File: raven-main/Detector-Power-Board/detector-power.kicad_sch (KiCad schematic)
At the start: 34 parts, among them J1 DeployLipo, J2 Conn_01x06, J9 UCLipo, U1 LM51571QRTERQ1, U7 TPS7A4701xRGW, U8 TPS7A4701xRGW

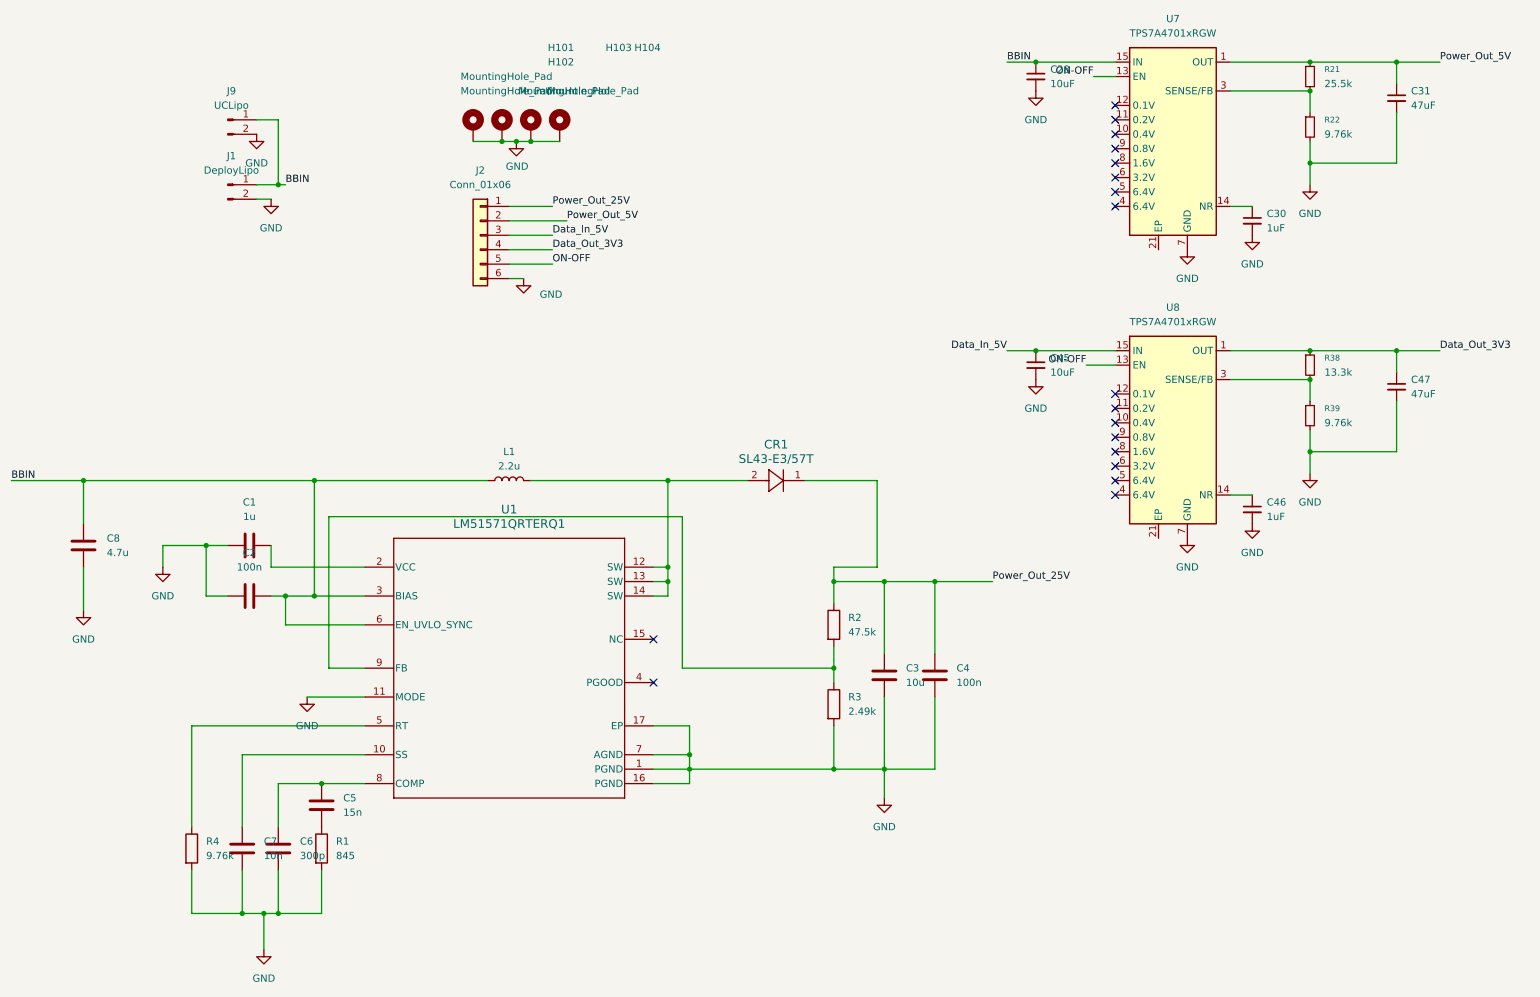
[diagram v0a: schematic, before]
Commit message: Updated power circuit
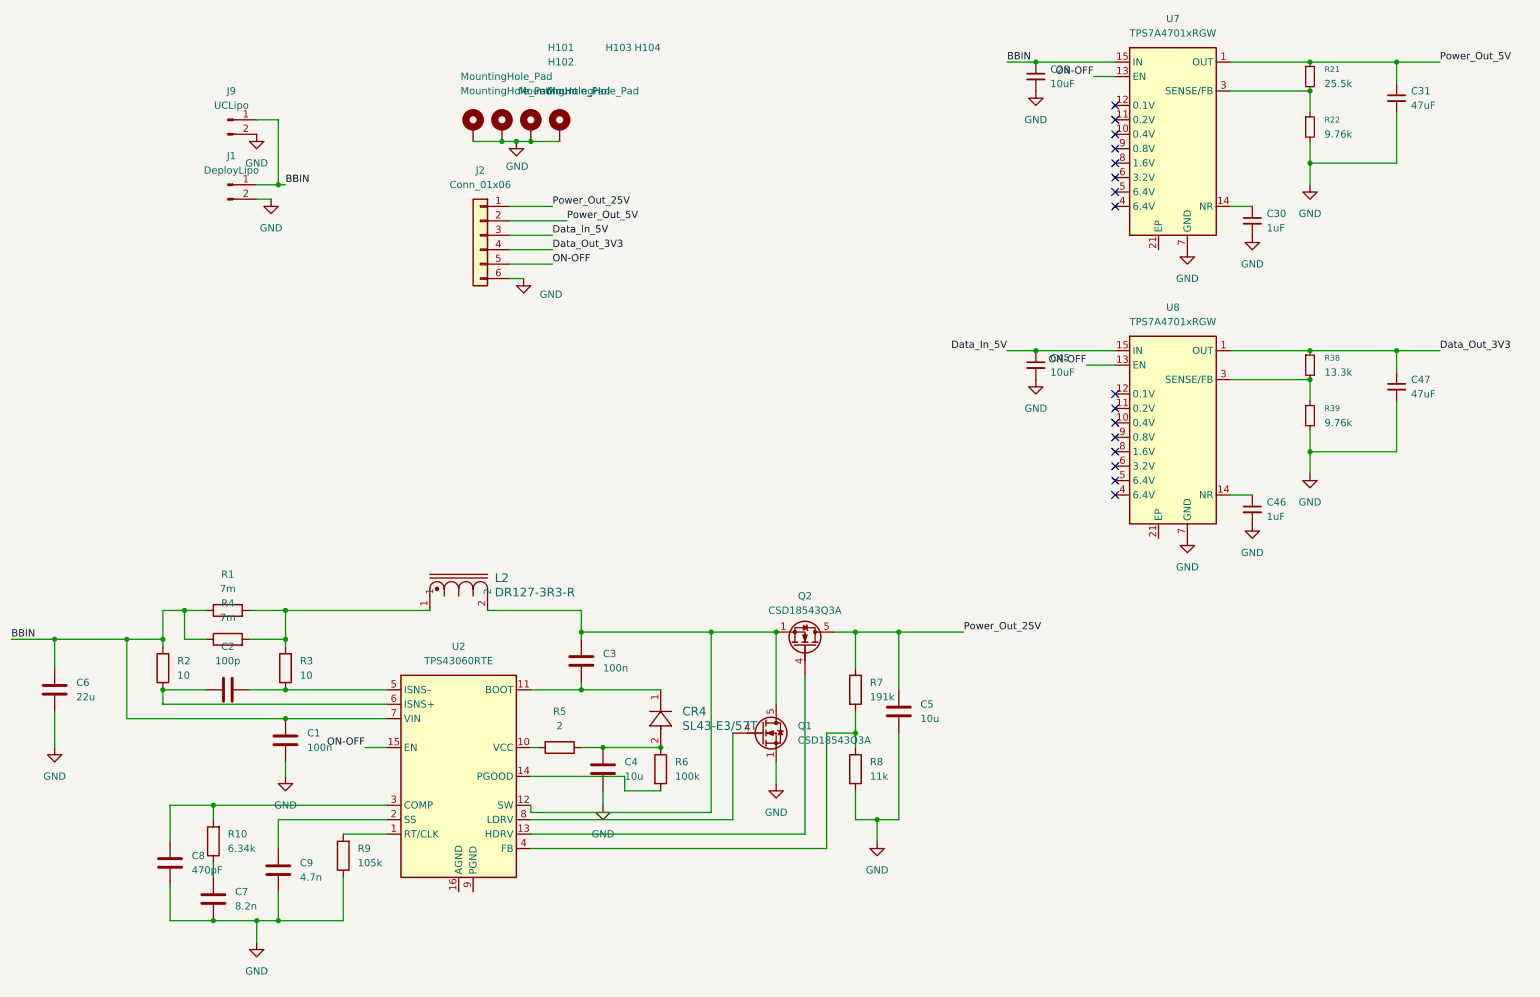
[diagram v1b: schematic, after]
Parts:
- removed CR1: SL43-E3/57T, SL43-E3-57T:DIODE_DO214AB, symbol 2026-08-05_22-06-24:SL43-E3_57T
- removed L1: 2.2u, Inductor_SMD:L_0402_1005Metric, symbol Device:L
- removed U1: LM51571QRTERQ1, LM51571QRTERQ1:RTE0016K, symbol 2026-08-05_21-30-25:LM51571QRTERQ1
- added C9: 4.7n, Capacitor_SMD:C_0402_1005Metric, symbol Device:C
- added CR4: SL43-E3/57T, SL43-E3-57T:DIODE_DO214AB, symbol 2026-08-05_22-06-24:SL43-E3_57T
- added L2: DR127-3R3-R, DR127-3R3-R:DR127, symbol DR127:DR127-3R3-R
- added Q1, Q2: CSD18543Q3A, Package_SON:VSON-8_3.3x3.3mm_P0.65mm_NexFET, symbol Transistor_FET:CSD18543Q3A
- added R10: 6.34k, Resistor_SMD:R_0402_1005Metric, symbol Device:R
- added R5: 2, Resistor_SMD:R_0402_1005Metric, symbol Device:R
- added R6: 100k, Resistor_SMD:R_0402_1005Metric, symbol Device:R
- added R7: 191k, Resistor_SMD:R_0402_1005Metric, symbol Device:R
- added R8: 11k, Resistor_SMD:R_0402_1005Metric, symbol Device:R
- added R9: 105k, Resistor_SMD:R_0402_1005Metric, symbol Device:R
- added U2: TPS43060RTE, Package_DFN_QFN:Texas_RTE_WQFN-16-1EP_3x3mm_P0.5mm_EP1.2x0.8mm_ThermalVias, symbol Converter_DCDC:TPS43060RTE
- C1: value 1u -> 100n
- C2: value 100n -> 100p
- C3: value 10u -> 100n
- C4: value 100n -> 10u
- C5: value 15n -> 10u
- C6: value 300p -> 22u
- C7: value 10n -> 8.2n
- C8: value 4.7u -> 470pF
- R1: value 845 -> 7m
- R2: value 47.5k -> 10
- R3: value 2.49k -> 10
- R4: value 9.76k -> 7m
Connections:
- net BBIN: now also C1.1, C6.1, R1.1, R2.2, R4.1, U2.7 (VIN); no longer C2.2, C8.2
- net GND: now also C1.2, C4.2, C5.2, C6.2, C7.2, C8.2, C9.2, Q1.1 (S), Q1.2 (S), Q1.3 (S), R8.2, R9.1; no longer C1.1, C2.1, C3.1, C4.1, C6.1, C7.1, C8.1, R1.2, R3.2, R4.2
- net ON-OFF: now also U2.15 (EN)
- net Power_Out_25V: now also C5.1, Q2.5 (D), R7.1; no longer C3.2, C4.2, R2.1
- net at R3.1: now also C2.2, U2.5 (ISNS–); no longer R2.2
- new net: C7.1, R10.1
- new net: C3.1, L2.2, Q1.5 (D), Q2.1 (S), Q2.2 (S), Q2.3 (S), U2.12 (SW)
- new net: C3.2, CR4.1, U2.11 (BOOT)
- new net: C9.1, U2.2 (SS)
- new net: C8.1, R10.2, U2.3 (COMP)
- new net: L2.1, R1.2, R3.2, R4.2
- new net: C4.1, CR4.2, R5.1, R6.1
- new net: Q1.4 (G), U2.8 (LDRV)
- new net: Q2.4 (G), U2.13 (HDRV)
- new net: R6.2, U2.14 (PGOOD)
- new net: C2.1, R2.1, U2.6 (ISNS+)
- new net: R7.2, R8.1, U2.4 (FB)
- new net: R9.2, U2.1 (RT/CLK)
- new net: R5.2, U2.10 (VCC)
- new net: U2.16 (AGND), U2.17 (AGND)
- no-connect marks 18 -> 16
